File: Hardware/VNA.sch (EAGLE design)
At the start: 413 parts, among them IC1 LTC5510, IC10 LT5560, IC11 LTC6362, IC12 MCP33131D-10-E/MS, IC13 SI5351C, IC14 MAX2871, IC15 NCP702-3.3, IC16 RFSW6042, IC17 AP2114H, IC18 RFSW6042, IC19 MAX2871, IC2 LT5560, IC20 NCP702-3.3, IC21 AP2114H, IC22 F2912, IC23 F1958, IC24 TRF37A73, IC25 F2912, IC26 F2912, IC27 F2912, IC28 LDL212PU50R, IC29 LDL212PU50R, IC3 LTC6362, IC30 LDL212PU50R, IC31 LDL212PU50R, IC32 TPS65265, IC33 STM32L432KC, IC34 NCP702-1.8, IC35 NCP702-1.8, IC36 NCP702-1.8, IC4 MCP33131D-10-E/MS, IC5 LTC5510, IC6 LT5560, IC7 LTC6362, IC8 MCP33131D-10-E/MS, IC9 LTC5510, J1 U.FL-R-SMT, J2 U.FL-R-SMT, J3 DCJ0202, Q1 FA-128 26MHz, T1 MABA011082, T2 MABA011082, T3 MABA011082, U2 6SLX9TQG144, U4 W25Q16BVSN, X1 RLB DUT/RF IN, X2 RLB DUT/RF IN, X3 MINI-USB-32005-201

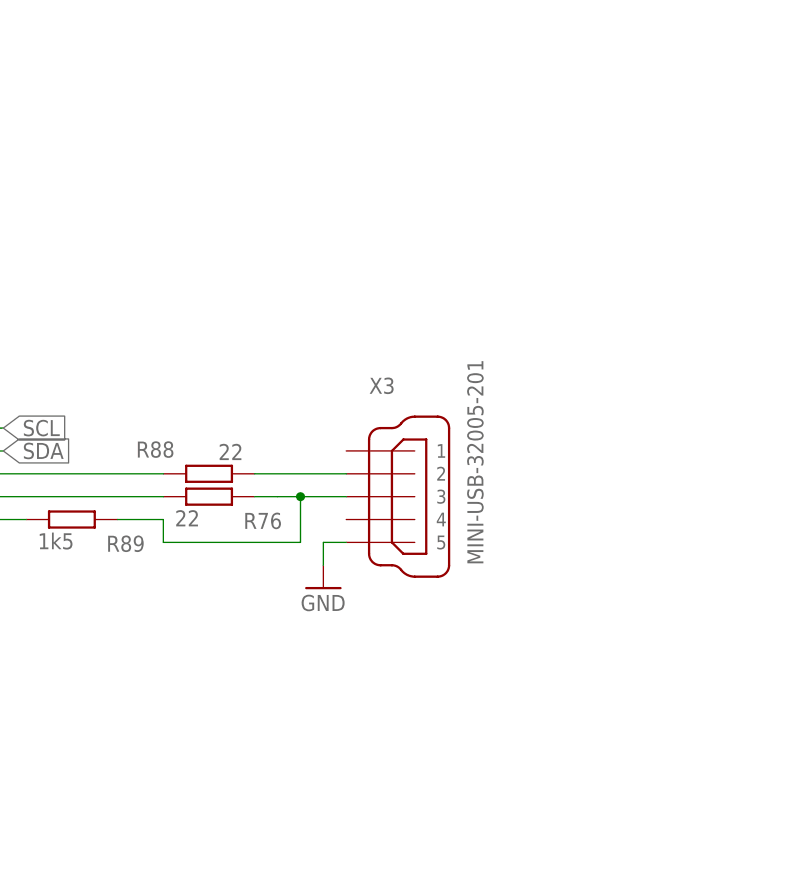
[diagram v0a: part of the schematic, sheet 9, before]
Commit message: Routing
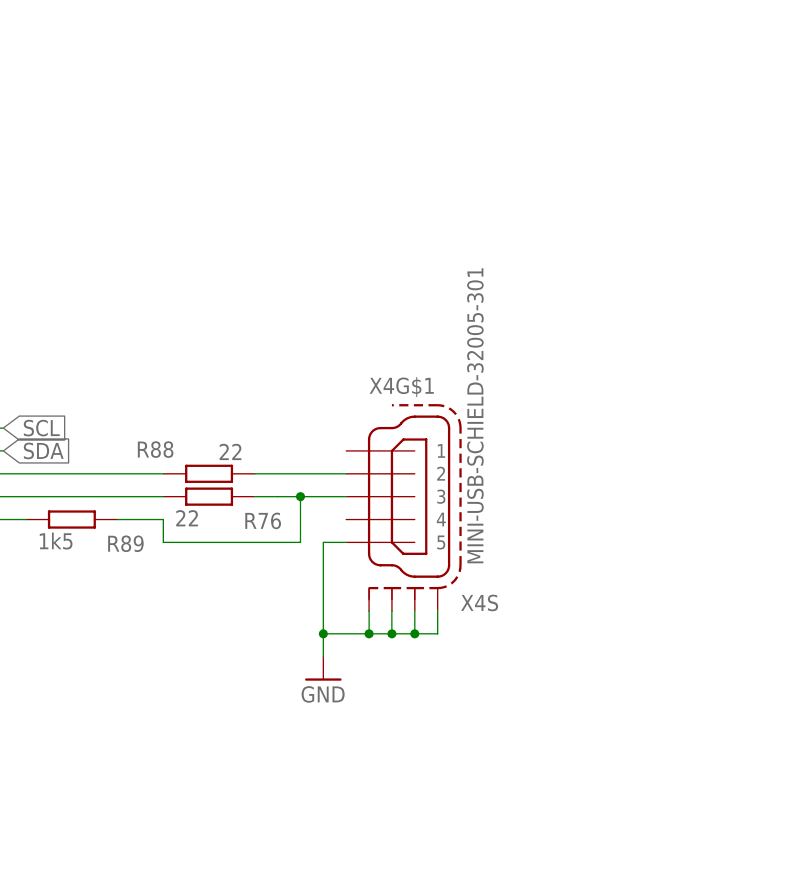
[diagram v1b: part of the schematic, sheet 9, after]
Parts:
- removed X3: MINI-USB-32005-201, con-cypressindustries:MINI-USB-32005-201
- added X4: MINI-USB-SCHIELD-32005-301, con-cypressindustries:MINI-USB-SCHIELD-32005-301
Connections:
- net GND: now also X4G$1.5, X4S.S1, X4S.S2, X4S.S3, X4S.S4; no longer X3.5
- net N$185: now also X4G$1.2; no longer X3.2
- net N$186: now also X4G$1.3; no longer X3.3
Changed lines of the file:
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@@
 <part name="GND212" library="supply1" deviceset="GND" device=""/>
 <part name="SUPPLY29" library="supply2" deviceset="+12V" device=""/>
-<part name="X3" library="con-cypressindustries" deviceset="MINI-USB-" device="32005-201"/>
 <part name="U2" library="xilinx_devices_V6" deviceset="6SLX9TQG144" device=""/>
 <part name="JTAG" library="con-ml" deviceset="ML10" device=""/>
@@
 <part name="SUPPLY21" library="supply2" deviceset="+5V/3" device=""/>
 <part name="SUPPLY14" library="supply2" deviceset="+5V/2" device=""/>
+<part name="X4" library="con-cypressindustries" deviceset="MINI-USB-SCHIELD-" device="32005-301"/>
 </parts>
 <sheets>
@@
 </plain>
 <instances>
-<instance part="X3" gate="G$1" x="223.52" y="66.04" smashed="yes">
-<attribute name="NAME" x="220.98" y="77.47" size="1.778" layer="95"/>
-<attribute name="VALUE" x="233.68" y="58.42" size="1.778" layer="96" rot="R90"/>
-</instance>
 <instance part="U2" gate="B2" x="327.66" y="190.5" smashed="yes" rot="MR0">
 <attribute name="NAME" x="327.66" y="231.902" size="1.778" layer="95"/>
@@
 <attribute name="VALUE" x="76.2" y="66.04" size="1.778" layer="96"/>
 </instance>
-<instance part="GND217" gate="1" x="215.9" y="55.88" smashed="yes">
-<attribute name="VALUE" x="213.36" y="53.34" size="1.778" layer="96"/>
+<instance part="GND217" gate="1" x="215.9" y="45.72" smashed="yes">
+<attribute name="VALUE" x="213.36" y="43.18" size="1.778" layer="96"/>
 </instance>
 <instance part="R76" gate="G$1" x="203.2" y="66.04" smashed="yes">
@@
 <attribute name="VALUE" x="50.8" y="81.28" size="1.778" layer="96"/>
 </instance>
+<instance part="X4" gate="G$1" x="223.52" y="66.04" smashed="yes">
+<attribute name="NAME" x="220.98" y="77.47" size="1.778" layer="95"/>
+<attribute name="VALUE" x="233.68" y="58.42" size="1.778" layer="96" rot="R90"/>
+</instance>
+<instance part="X4" gate="S" x="223.52" y="55.88" smashed="yes">
+<attribute name="NAME" x="231.14" y="53.34" size="1.778" layer="95"/>
+</instance>
 </instances>
 <busses>
@@
 </segment>
 <segment>
-<pinref part="X3" gate="G$1" pin="5"/>
 <pinref part="GND217" gate="1" pin="GND"/>
 <wire x1="218.44" y1="60.96" x2="215.9" y2="60.96" width="0.1524" layer="91"/>
-<wire x1="215.9" y1="60.96" x2="215.9" y2="58.42" width="0.1524" layer="91"/>
+<wire x1="215.9" y1="60.96" x2="215.9" y2="50.8" width="0.1524" layer="91"/>
+<pinref part="X4" gate="G$1" pin="5"/>
+<pinref part="X4" gate="S" pin="S4"/>
+<wire x1="215.9" y1="50.8" x2="215.9" y2="48.26" width="0.1524" layer="91"/>
+<wire x1="215.9" y1="50.8" x2="220.98" y2="50.8" width="0.1524" layer="91"/>
+<wire x1="220.98" y1="50.8" x2="223.52" y2="50.8" width="0.1524" layer="91"/>
+<wire x1="223.52" y1="50.8" x2="226.06" y2="50.8" width="0.1524" layer="91"/>
+<wire x1="226.06" y1="50.8" x2="228.6" y2="50.8" width="0.1524" layer="91"/>
+<wire x1="228.6" y1="50.8" x2="228.6" y2="53.34" width="0.1524" layer="91"/>
+<junction x="215.9" y="50.8"/>
+<pinref part="X4" gate="S" pin="S3"/>
+<wire x1="226.06" y1="53.34" x2="226.06" y2="50.8" width="0.1524" layer="91"/>
+<junction x="226.06" y="50.8"/>
+<pinref part="X4" gate="S" pin="S2"/>
+<wire x1="223.52" y1="53.34" x2="223.52" y2="50.8" width="0.1524" layer="91"/>
+<junction x="223.52" y="50.8"/>
+<pinref part="X4" gate="S" pin="S1"/>
+<wire x1="220.98" y1="53.34" x2="220.98" y2="50.8" width="0.1524" layer="91"/>
+<junction x="220.98" y="50.8"/>
 </segment>
 <segment>
@@
 <net name="N$185" class="0">
 <segment>
-<pinref part="X3" gate="G$1" pin="2"/>
 <pinref part="R88" gate="G$1" pin="1"/>
 <wire x1="218.44" y1="68.58" x2="208.28" y2="68.58" width="0.1524" layer="91"/>
+<pinref part="X4" gate="G$1" pin="2"/>
 </segment>
 </net>
 <net name="N$186" class="0">
 <segment>
-<pinref part="X3" gate="G$1" pin="3"/>
 <pinref part="R76" gate="G$1" pin="2"/>
 <wire x1="218.44" y1="66.04" x2="213.36" y2="66.04" width="0.1524" layer="91"/>
@@
 <wire x1="213.36" y1="60.96" x2="213.36" y2="66.04" width="0.1524" layer="91"/>
 <junction x="213.36" y="66.04"/>
+<pinref part="X4" gate="G$1" pin="3"/>
 </segment>
 </net>
